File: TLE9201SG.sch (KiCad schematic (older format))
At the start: 7 parts, among them U4 TLE9201SG

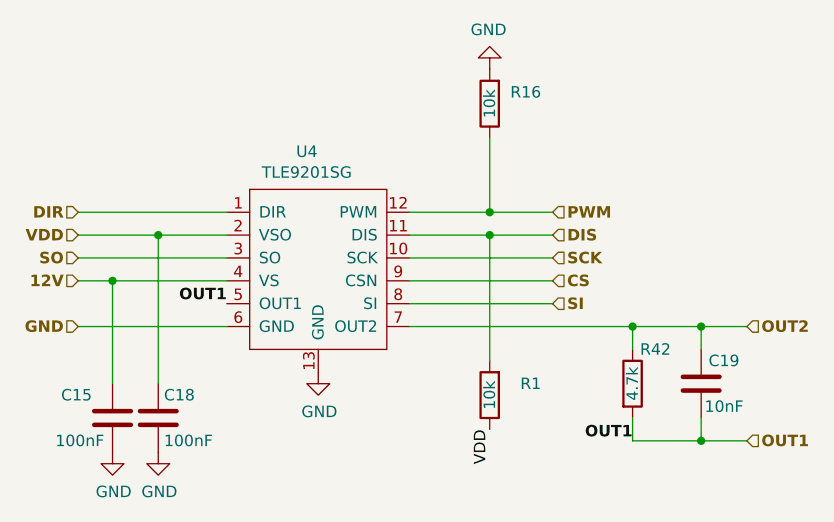
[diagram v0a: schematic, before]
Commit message: R0.3 released
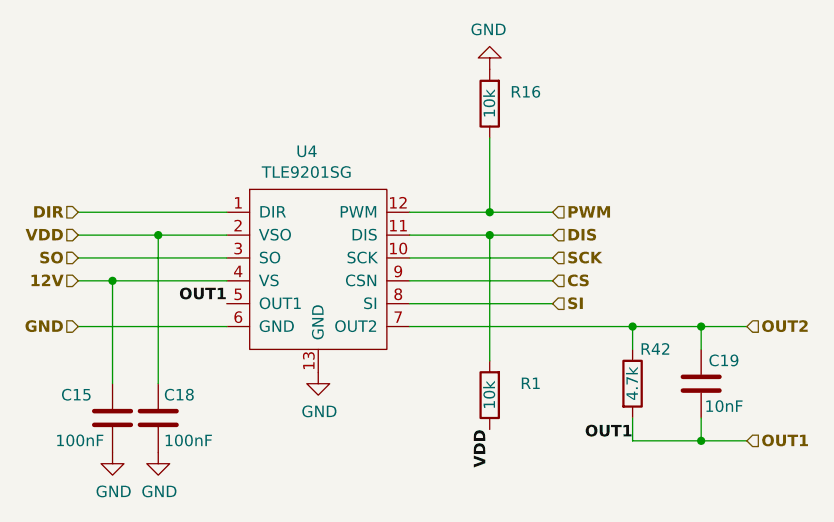
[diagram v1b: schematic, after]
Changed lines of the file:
@@
 Wire Wire Line
 	4675 3350 5025 3350
-Text Label 6475 4200 3    50   ~ 0
+Text Label 6475 4200 3    50   ~ 6
 VDD
 Wire Wire Line
